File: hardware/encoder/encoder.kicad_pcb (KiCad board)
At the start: 4 copper layers, 32 x 14 mm, 7 parts, among them J1 Conn_01x06, U1 MT6701CT, U2 SMF5.0CA

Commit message: update rfBat firmware
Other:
- copper layers 4 -> 2
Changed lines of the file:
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@@
 	(layers
 		(0 "F.Cu" signal)
-		(1 "In1.Cu" signal)
-		(2 "In2.Cu" signal)
 		(31 "B.Cu" signal)
 		(32 "B.Adhes" user "B.Adhesive")
@@
 			)
 			(layer "dielectric 1"
-				(type "prepreg")
-				(thickness 0.1)
+				(type "core")
+				(thickness 1.51)
 				(material "FR4")
 				(epsilon_r 4.5)
-				(loss_tangent 0.02)
-			)
-			(layer "In1.Cu"
-				(type "copper")
-				(thickness 0.035)
-			)
-			(layer "dielectric 2"
-				(type "core")
-				(thickness 1.24)
-				(material "FR4")
-				(epsilon_r 4.5)
-				(loss_tangent 0.02)
-			)
-			(layer "In2.Cu"
-				(type "copper")
-				(thickness 0.035)
-			)
-			(layer "dielectric 3"
-				(type "prepreg")
-				(thickness 0.1)
-				(material "FR4")
-				(epsilon_r 4.5)

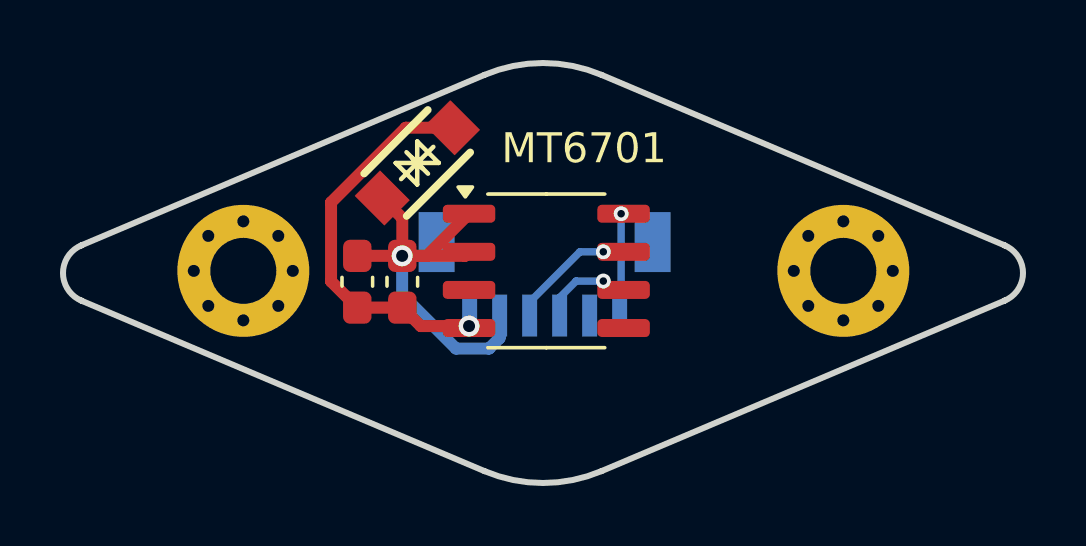
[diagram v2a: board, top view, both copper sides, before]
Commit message: update rfBat pcb
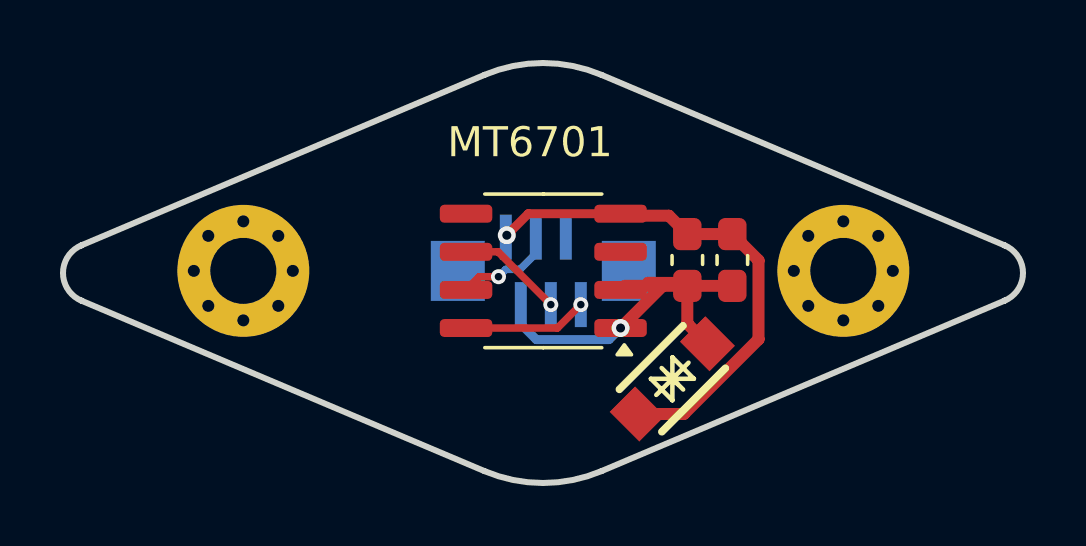
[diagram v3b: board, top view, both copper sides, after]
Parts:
- J1: footprint encoder:CONN-SMD_6P-P1.00_BX-SH1.0-6PLT -> encoder:FPC-SMD_6P-P0.50_HDGC_0.5K-A-6PB
- moved C3 12.5 mm to (206.6, 74.3), turned to 90 degrees
- moved U2 11.1 mm to (204.6, 78.3), turned to -135 degrees
- moved C2 9.53 mm to (205.1, 74.3), turned to 90 degrees
- moved J1 0.27 mm to (200.3, 74.7), turned to 0 degrees
- moved U1 0.10 mm to (200.3, 74.7), turned to 180 degrees
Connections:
- J1 pad 1: /CSN -> GND
- J1 pad 2: /MOSI -> +3V3
- J1 pad 3: /MISO -> /CLK
- J1 pad 4: /CLK -> /MISO
- J1 pad 5: +3V3 -> /MOSI
- J1 pad 6: GND -> /CSN
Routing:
- net GND: track 13.3 -> 17.0 mm
- net +3V3: track 15.0 -> 12.9 mm
- net /CSN: track 3.42 -> 4.15 mm
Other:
- board text removed: "C"
- board text removed: "I"
- board text removed: "O"
- board text removed: "S"
- board text removed: "V"
